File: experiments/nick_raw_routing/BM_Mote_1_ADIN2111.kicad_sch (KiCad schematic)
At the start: 36 parts, among them U1 ADIN2111BCPZ, U2 AP22913CN4-7, U3 AP22913CN4-7, Y1 ABM11W-25.0000MHZ-6-K1Z-T3

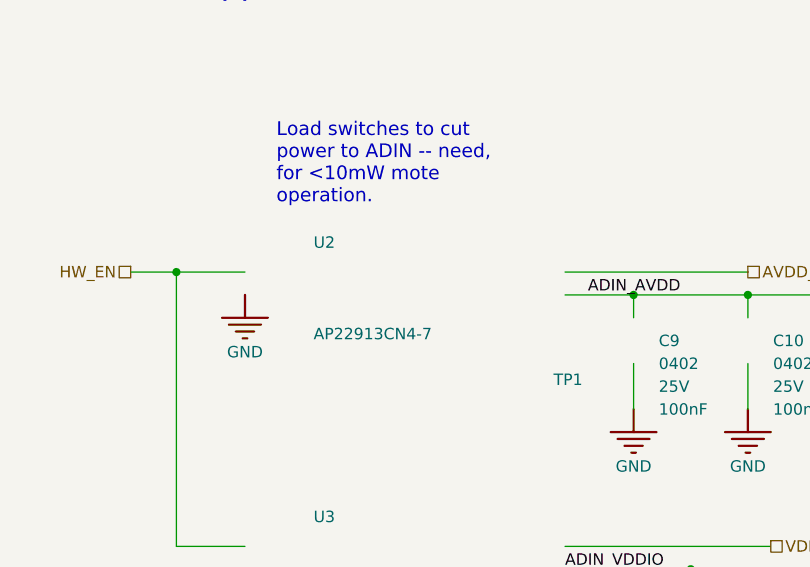
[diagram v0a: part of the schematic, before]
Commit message: updates before the sofar review
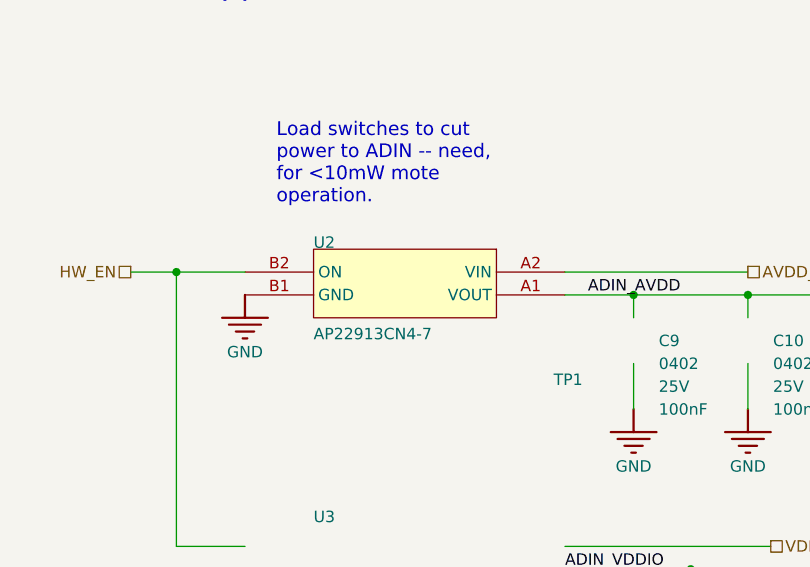
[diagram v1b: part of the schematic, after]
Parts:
- U1: PLANNED LCSC (none) -> none shown yet; check My Parts; SOURCING JLC global sourcing (D26); no LCSC listing, DK 120 -> Bought: JLC global sourcing DOB202610190524705 (2026-10-18)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
- U2: SOURCING JLC global sourcing, all 40 (LCSC has 30) (D26) -> Bought: JLC global sourcing DOB202610190524705 (2026-10-18)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
- Y1: PLANNED LCSC (none) -> none shown yet; SOURCING JLC global sourcing (D26); no LCSC listing, DK 87 -> Bought: JLC global sourcing DOB202610190524705 (2026-10-18)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
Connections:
- net ADIN_AVDD: now also U2.A1 (VOUT)
- net AVDD_H + AVDD_L: now also U2.A2 (VIN)
- net GND: now also U2.B1 (GND)
- net HW_EN: now also U2.B2 (ON)
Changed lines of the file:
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@@
 			)
 		)
-		(property "SOURCING" "JLC global sourcing (D26); no LCSC listing, DK 120"
+		(property "SOURCING" "Bought: JLC global sourcing DOB202610190524705 (2026-10-18), qty 22, ready 2026-11-05"
 			(at 187.96 204.47 0)
 			(hide yes)
@@
 			)
 		)
-		(property "PLANNED LCSC" ""
+		(property "PLANNED LCSC" "none shown yet; check My Parts"
 			(at 187.96 204.47 0)
 			(hide yes)
@@
 			)
 		)
+		(property "Field12" ""
+			(at 187.96 204.47 0)
+			(hide yes)
+			(show_name no)
+			(do_not_autoplace no)
+			(effects
+				(font
+					(size 1.27 1.27)
+				)
+			)
+		)
 		(pin "2"
 		)
@@
 		(lib_id "BM_Mote_000639-AB-altium-import:ADIN_2_AP22913CN4-7-Symbol-1_Sofar Ocean Technologies, Inc.")
 		(at 106.68 199.39 0)
-		(unit 0)
+		(unit 1)
 		(body_style 1)
 		(exclude_from_sim no)
@@
 			)
 		)
-		(property "SOURCING" "JLC global sourcing, all 40 (LCSC has 30) (D26)"
+		(property "SOURCING" "Bought: JLC global sourcing DOB202610190524705 (2026-10-18), qty 42, ready 2026-11-05"
 			(at 106.68 199.39 0)
 			(hide yes)
@@
 				(path "/30e82bf5-1344-486b-817c-02d3b0649ce4/3c398828-e355-49f6-be37-cb3640d2c671/6b1c7de5-1c82-42d9-9a95-c340ffb1bf15"
 					(reference "U2")
-					(unit 0)
+					(unit 1)
 				)
 			)
@@
 			)
 		)
-		(property "SOURCING" "JLC global sourcing (D26); no LCSC listing, DK 120"
+		(property "SOURCING" "Bought: JLC global sourcing DOB202610190524705 (2026-10-18), qty 22, ready 2026-11-05"
 			(at 123.19 85.2678 0)
 			(hide yes)
@@
 			)
 		)
-		(property "PLANNED LCSC" ""
+		(property "PLANNED LCSC" "none shown yet; check My Parts"
 			(at 123.19 85.2678 0)
 			(hide yes)
@@
 			)
 		)
+		(property "Field12" ""
+			(at 123.19 85.2678 0)
+			(hide yes)
+			(show_name no)
+			(do_not_autoplace no)
+			(effects
+				(font
+					(size 1.27 1.27)
+				)
+			)
+		)
 		(pin "48"
 		)
@@
 			)
 		)
-		(property "SOURCING" "JLC global sourcing (D26); no LCSC listing, DK 87"
+		(property "SOURCING" "Bought: JLC global sourcing DOB202610190524705 (2026-10-18), qty 22, ready 2026-11-05"
 			(at 176.53 118.11 0)
 			(hide yes)
@@
 			)
 		)
-		(property "PLANNED LCSC" ""
+		(property "PLANNED LCSC" "none shown yet"
 			(at 176.53 118.11 0)
 			(hide yes)
